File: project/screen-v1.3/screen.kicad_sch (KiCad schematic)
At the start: 37 parts, among them J1 TTL-connect-pin4, J2 USB_C_6pin, J3 Conn_01x02_Female, Q1 S8050, SW1 SW_DPDT_x2, SW2 SW_Push, SW3 SW_Push, U1 SPX3819M5-L-3-3, U2 ESP-12E, U3 TFT_1.3_12, U4 TP4056_[C16581]

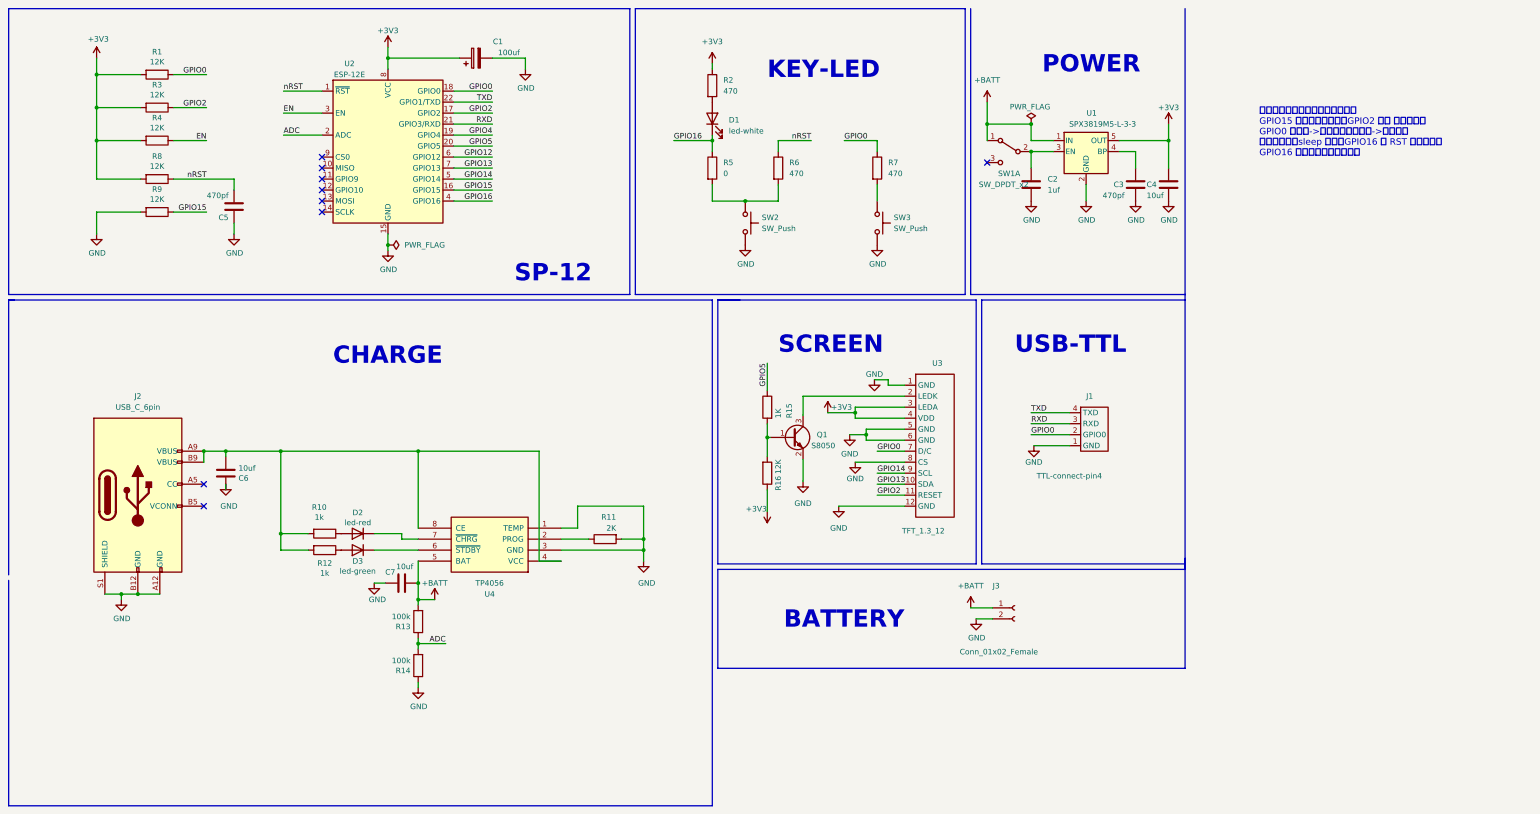
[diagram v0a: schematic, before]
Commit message: update screen v1.3
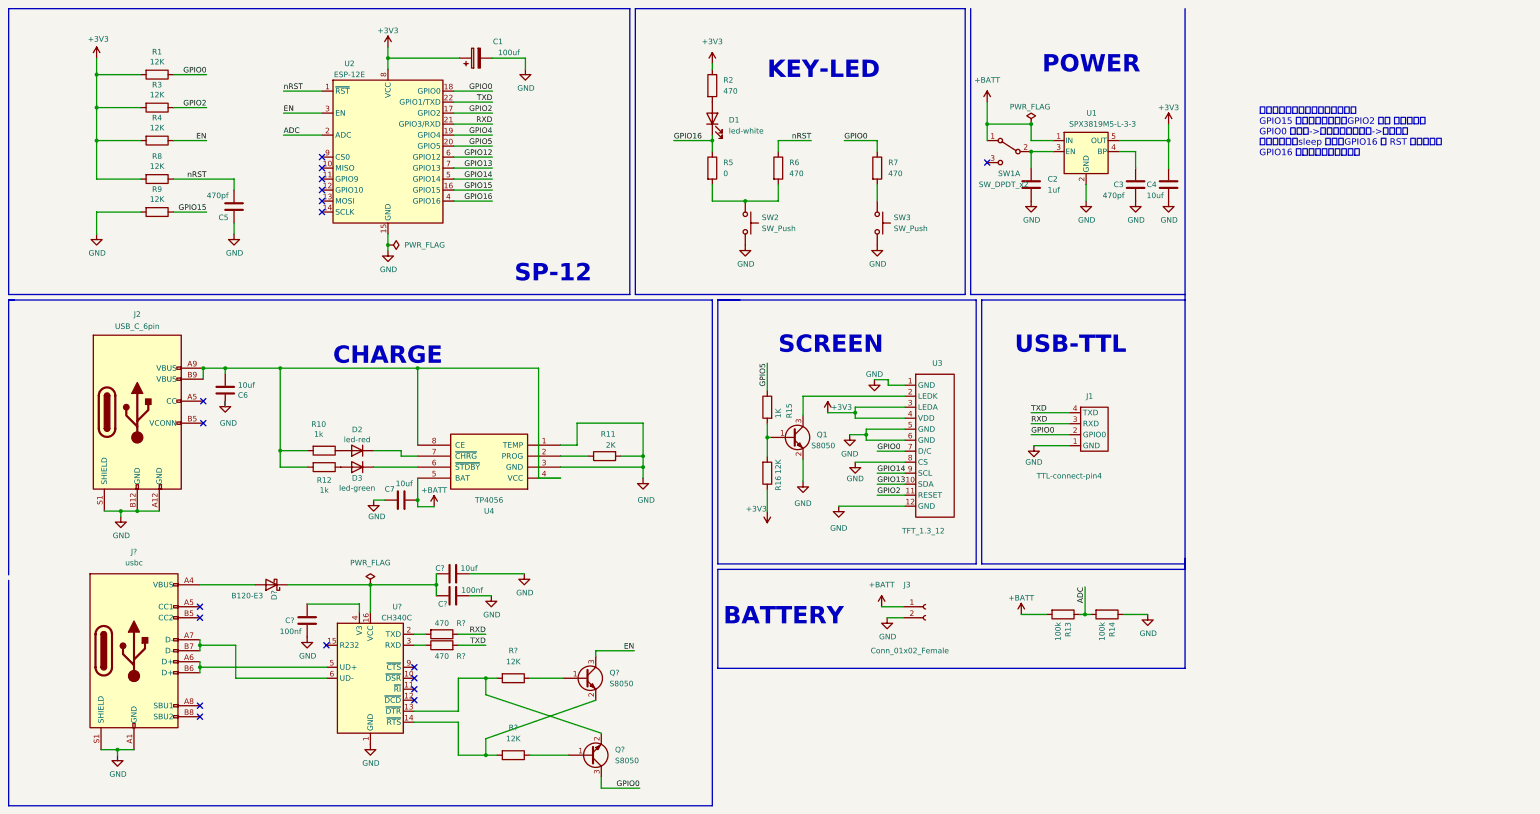
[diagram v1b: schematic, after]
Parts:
- added C?: 10uf, Capacitor_SMD:C_0402_1005Metric, symbol Device:C
- added C? (x2): 100nf, Capacitor_SMD:C_0402_1005Metric, symbol Device:C
- added D?: B120-E3, Diode_SMD:D_SOD-123, symbol Diode:B120-E3
- added J?: usbc, Connector_USB:USB_C_Receptacle_HRO_TYPE-C-31-M-12, symbol Connector:USB_C_Receptacle_USB2.0
- added Q? (x2): S8050, Package_TO_SOT_SMD:TSOT-23, symbol Device:Q_NPN_BEC
- added R? (x2): 12K, Resistor_SMD:R_0402_1005Metric, symbol Device:R
- added R? (x2): 470, Resistor_SMD:R_0402_1005Metric, symbol Device:R
- added U?: CH340C, lc_lib:SOP-16_150MIL, symbol Interface_USB:CH340C
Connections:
- net EN: now also Q?.3 (C)
- net GND: now also C?.2, C?.2, C?.2, J?.A1 (GND), J?.A12 (GND), J?.B1 (GND), J?.B12 (GND), J?.S1 (SHIELD), U?.1 (GND)
- net GPIO0: now also Q?.3 (C)
- net RXD: now also R?.1
- net TXD: now also R?.2
- new net: Q?.1 (B), R?.1 (x2)
- new net: Q?.2 (E), R?.2, U?.14 (~{RTS})
- new net: Q?.2 (E), R?.2, U?.13 (~{DTR})
- new net: C?.1, C?.1, D?.1 (K), U?.16 (VCC)
- new net: R?.2, U?.2 (TXD)
- new net: R?.1, U?.3 (RXD)
- new net: C?.1, U?.4 (V3)
- new net: J?.A6 (D+), J?.B6 (D+), U?.5 (UD+)
- new net: J?.A7 (D-), J?.B7 (D-), U?.6 (UD-)
- new net: D?.2 (A), J?.A4 (VBUS), J?.A9 (VBUS), J?.B4 (VBUS), J?.B9 (VBUS)
- no-connect marks 9 -> 18
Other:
- moved on the sheet: C6, C7, D2, D3, J2, J3, R10, R11, R12, R13, R14, U4
